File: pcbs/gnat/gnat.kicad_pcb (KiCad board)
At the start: 2 copper layers, 119.7 x 84.2 mm, 19 parts, among them SW1 SW_PUSH, SW10 SW_PUSH, SW11 SW_PUSH, SW12 SW_PUSH, SW13 SW_PUSH, SW14 SW_PUSH, SW15 SW_PUSH, SW16 SW_PUSH, SW2 SW_PUSH, SW3 SW_PUSH, SW4 SW_PUSH, SW5 SW_PUSH, SW6 SW_PUSH, SW7 SW_PUSH, SW8 SW_PUSH, SW9 SW_PUSH, U1 ProMicro

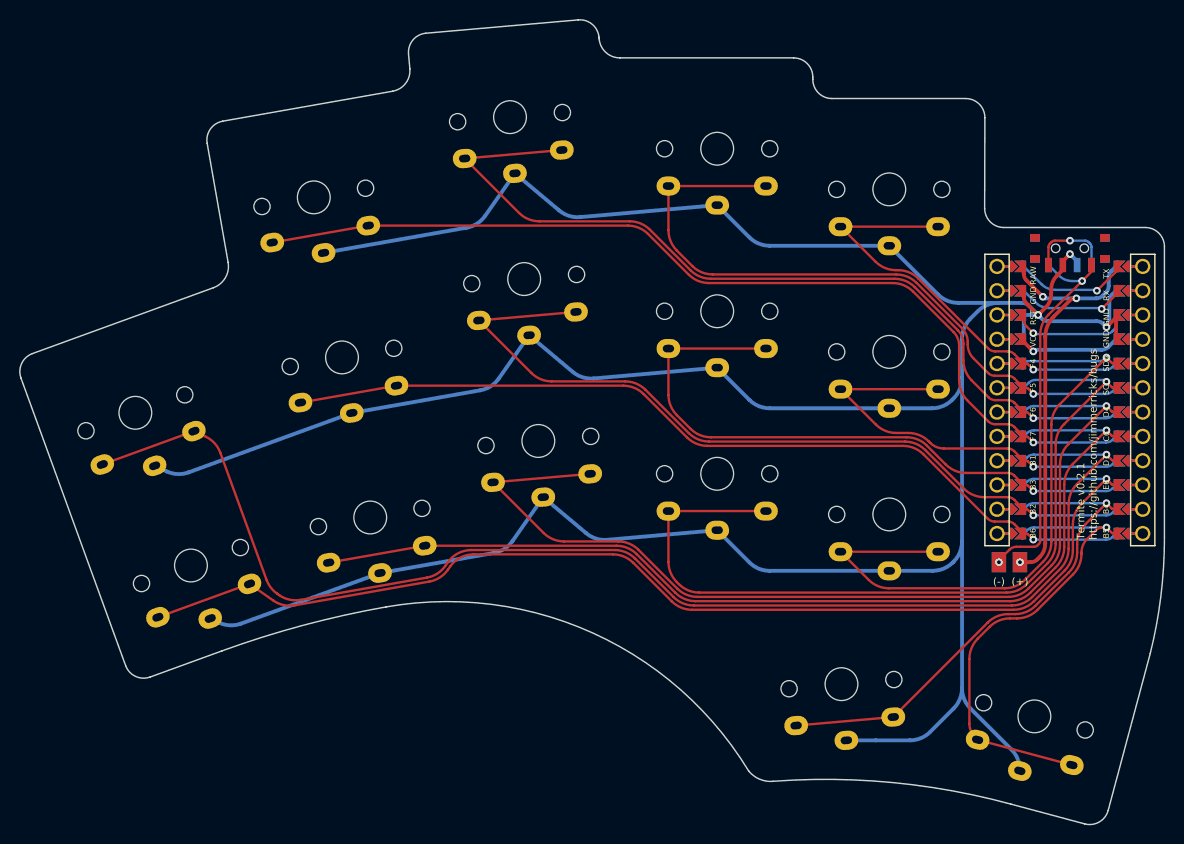
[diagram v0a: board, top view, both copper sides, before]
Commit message: Update gnat & mosquito edge
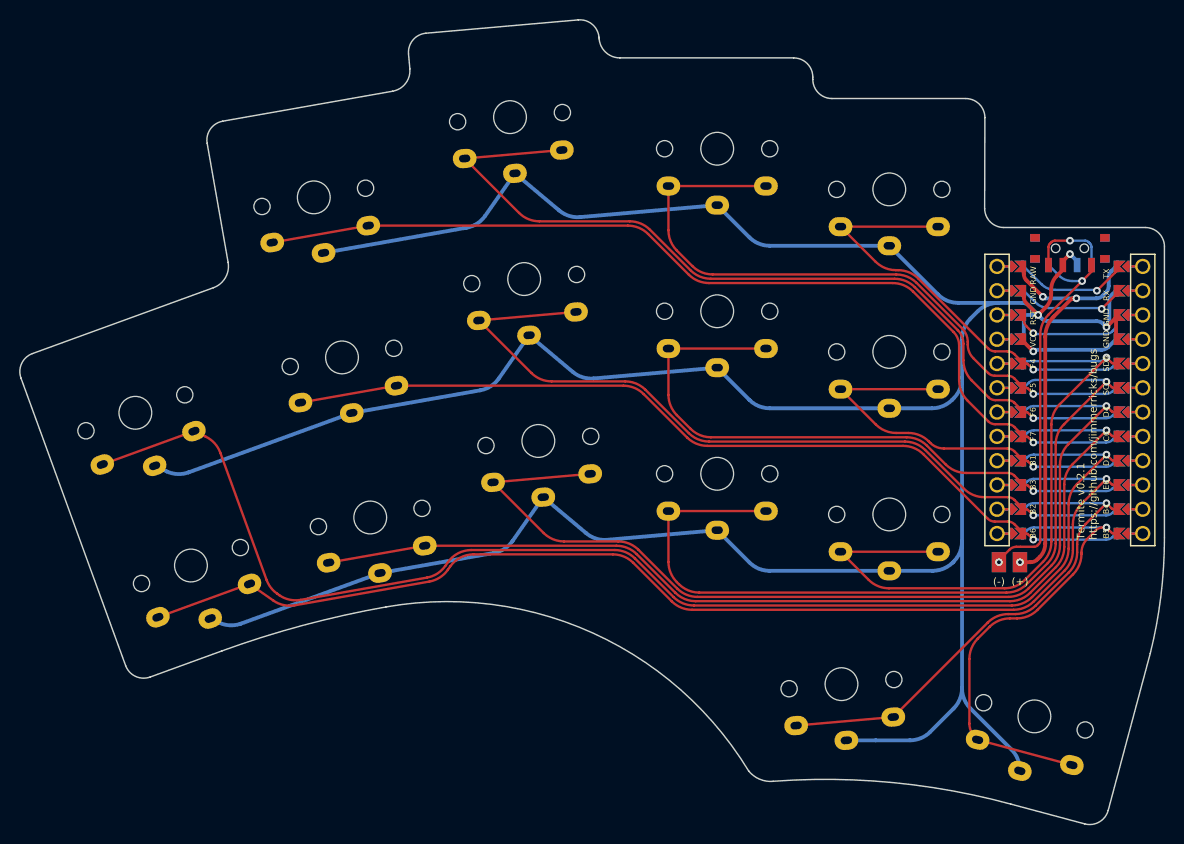
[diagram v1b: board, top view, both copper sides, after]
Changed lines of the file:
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@@
-(kicad_pcb (version 20210925) (generator pcbnew)
+(kicad_pcb (version 20211014) (generator pcbnew)
   (general
     (thickness 1.6)
@@
     )
   )
-  (gr_arc (start 85.545766 205.46248) (end 67.853328 105.132673) (angle -9.999121664) (layer "Edge.Cuts") (width 0.15))
+  (gr_arc (start 50.701495 109.728634) (mid 59.177088 107.056254) (end 67.853328 105.132673) (layer "Edge.Cuts") (width 0.15))
   (gr_line (start 30.870328 78.635657) (end 49.806346 71.743508) (layer "Edge.Cuts") (width 0.15))
   (gr_line (start 50.701495 109.728636) (end 43.183183 112.464287) (layer "Edge.Cuts") (width 0.15))
-  (gr_arc (start 72.200655 47.117941) (end 72.026343 45.125546) (angle -90) (layer "Edge.Cuts") (width 0.15))
-  (gr_arc (start 99.35345 97.913162) (end 147.791847 109.99194) (angle -14.00185829) (layer "Edge.Cuts") (width 0.15))
-  (gr_arc (start 147.275269 67.44594) (end 149.275272 67.445943) (angle -90) (layer "Edge.Cuts") (width 0.15))
+  (gr_arc (start 70.20826 47.292253) (mid 70.668562 45.832362) (end 72.026343 45.125546) (layer "Edge.Cuts") (width 0.15))
+  (gr_arc (start 149.27514 97.913221) (mid 148.902925 103.997948) (end 147.791847 109.99194) (layer "Edge.Cuts") (width 0.15))
+  (gr_arc (start 147.275272 65.445937) (mid 148.689487 66.031726) (end 149.275272 67.445943) (layer "Edge.Cuts") (width 0.15))
   (gr_line (start 112.494884 49.706792) (end 112.495279 49.955936) (layer "Edge.Cuts") (width 0.15))
-  (gr_line (start 133.214281 125.755736) (end 140.941679 127.826285) (layer "Edge.Cuts") (width 0.15))
+  (gr_line (start 133.214275 125.755733) (end 140.941679 127.826285) (layer "Edge.Cuts") (width 0.15))
   (gr_line (start 90.13216 45.549137) (end 90.146627 45.714507) (layer "Edge.Cuts") (width 0.15))
-  (gr_arc (start 51.118287 56.296082) (end 50.770987 54.326467) (angle -90) (layer "Edge.Cuts") (width 0.15))
-  (gr_arc (start 68.174652 49.041445) (end 68.553662 51.190899) (angle -84.99985992) (layer "Edge.Cuts") (width 0.15))
-  (gr_line (start 132.469399 65.445933) (end 147.275272 65.445947) (layer "Edge.Cuts") (width 0.15))
-  (gr_arc (start 113.817045 197.142315) (end 108.351573 123.36952) (angle 19.43846695) (layer "Edge.Cuts") (width 0.15))
-  (gr_arc (start 31.554358 80.51505) (end 30.870328 78.635657) (angle -90) (layer "Edge.Cuts") (width 0.15))
-  (gr_line (start 114.495282 51.955942) (end 128.49506 51.956155) (layer "Edge.Cuts") (width 0.15))
-  (gr_arc (start 141.459322 125.894435) (end 140.941679 127.826285) (angle -90) (layer "Edge.Cuts") (width 0.15))
-  (gr_line (start 143.391173 126.412071) (end 147.791847 109.99194) (layer "Edge.Cuts") (width 0.15))
-  (gr_arc (start 128.49506 53.956159) (end 130.495061 53.956158) (angle -90) (layer "Edge.Cuts") (width 0.15))
-  (gr_arc (start 42.499142 110.5849) (end 40.619755 111.268942) (angle -90) (layer "Edge.Cuts") (width 0.15))
+  (gr_arc (start 49.148672 56.643382) (mid 49.479981 55.148932) (end 50.770987 54.326467) (layer "Edge.Cuts") (width 0.15))
+  (gr_arc (start 70.34896 48.85122) (mid 69.906236 50.370135) (end 68.553662 51.190899) (layer "Edge.Cuts") (width 0.15))
+  (gr_line (start 132.469406 65.445944) (end 147.275272 65.445937) (layer "Edge.Cuts") (width 0.15))
+  (gr_arc (start 108.351573 123.36952) (mid 120.884362 123.505709) (end 133.214275 125.755733) (layer "Edge.Cuts") (width 0.15))
+  (gr_arc (start 29.674965 81.19908) (mid 29.741744 79.669801) (end 30.870328 78.635657) (layer "Edge.Cuts") (width 0.15))
+  (gr_line (start 114.495269 51.955938) (end 128.49506 51.956155) (layer "Edge.Cuts") (width 0.15))
+  (gr_arc (start 143.391172 126.412078) (mid 142.459317 127.626488) (end 140.941679 127.826285) (layer "Edge.Cuts") (width 0.15))
+  (gr_line (start 143.391172 126.412078) (end 147.791847 109.99194) (layer "Edge.Cuts") (width 0.15))
+  (gr_arc (start 128.495059 51.956158) (mid 129.909274 52.541944) (end 130.495061 53.956158) (layer "Edge.Cuts") (width 0.15))
+  (gr_arc (start 43.183184 112.464287) (mid 41.653905 112.397518) (end 40.619755 111.268942) (layer "Edge.Cuts") (width 0.15))
   (gr_line (start 149.275272 67.445943) (end 149.275145 97.913218) (layer "Edge.Cuts") (width 0.15))
-  (gr_arc (start 114.495275 49.955942) (end 112.495279 49.955936) (angle -90) (layer "Edge.Cuts") (width 0.15))
-  (gr_line (start 92.320939 47.706891) (end 110.494885 47.706788) (layer "Edge.Cuts") (width 0.15))
-  (gr_arc (start 108.092905 120.413812) (end 105.785147 122.286285) (angle -55.94629929) (layer "Edge.Cuts") (width 0.15))
-  (gr_arc (start 92.320931 45.524275) (end 90.146627 45.714507) (angle -85.00013873) (layer "Edge.Cuts") (width 0.15))
+  (gr_arc (start 114.495269 51.955938) (mid 113.08106 51.370148) (end 112.495279 49.955936) (layer "Edge.Cuts") (width 0.15))
+  (gr_line (start 92.320941 47.706885) (end 110.494894 47.706788) (layer "Edge.Cuts") (width 0.15))
+  (gr_arc (start 108.351999 123.374348) (mid 106.933066 123.149991) (end 105.785147 122.286285) (layer "Edge.Cuts") (width 0.15))
+  (gr_arc (start 92.320941 47.706885) (mid 90.846387 47.133469) (end 90.146627 45.714507) (layer "Edge.Cuts") (width 0.15))
   (gr_line (start 51.338431 69.089856) (end 49.148665 56.643377) (layer "Edge.Cuts") (width 0.15))
-  (gr_arc (start 48.991138 69.503748) (end 49.806346 71.743508) (angle -79.99998711) (layer "Edge.Cuts") (width 0.15))
-  (gr_arc (start 88.139767 45.723447) (end 90.13216 45.549137) (angle -90) (layer "Edge.Cuts") (width 0.15))
+  (gr_arc (start 51.33843 69.089856) (mid 51.055313 70.695498) (end 49.806346 71.743508) (layer "Edge.Cuts") (width 0.15))
+  (gr_arc (start 87.965457 43.731054) (mid 89.425346 44.191357) (end 90.13216 45.549137) (layer "Edge.Cuts") (width 0.15))
   (gr_line (start 29.674964 81.199082) (end 40.619755 111.268942) (layer "Edge.Cuts") (width 0.15))
-  (gr_arc (start 74.261808 141.477749) (end 105.785147 122.286285) (angle -68.66666424) (layer "Edge.Cuts") (width 0.15))
-  (gr_line (start 70.208269 47.292251) (end 70.348963 48.851219) (layer "Edge.Cuts") (width 0.15))
+  (gr_arc (start 67.853326 105.132673) (mid 89.468734 107.850638) (end 105.785147 122.286285) (layer "Edge.Cuts") (width 0.15))
+  (gr_line (start 70.20826 47.292253) (end 70.34896 48.85122) (layer "Edge.Cuts") (width 0.15))
   (gr_line (start 72.026343 45.125546) (end 87.965461 43.731057) (layer "Edge.Cuts") (width 0.15))
   (gr_line (start 50.770987 54.326467) (end 68.553662 51.190899) (layer "Edge.Cuts") (width 0.15))
-  (gr_arc (start 110.494887 49.706785) (end 112.494884 49.706792) (angle -90) (layer "Edge.Cuts") (width 0.15))
+  (gr_arc (start 110.494894 47.706788) (mid 111.909103 48.292579) (end 112.494884 49.706792) (layer "Edge.Cuts") (width 0.15))
   (gr_line (start 130.495061 53.956158) (end 130.469401 63.445945) (layer "Edge.Cuts") (width 0.15))
-  (gr_arc (start 132.469403 63.445942) (end 130.469401 63.445945) (angle -90) (layer "Edge.Cuts") (width 0.15))
+  (gr_arc (start 132.469406 65.445944) (mid 131.05519 64.860159) (end 130.469401 63.445945) (layer "Edge.Cuts") (width 0.15))
   (gr_text "Termite v0.2.1\nhttps://github.com/jimmerricks/bugs" (at 141.170001 74.890001 90) (layer "B.SilkS")
     (effects (font (size 0.8 0.8) (thickness 0.1)) (justify left mirror))
